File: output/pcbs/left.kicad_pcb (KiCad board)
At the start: 2 copper layers, 132 x 103 mm, 45 parts

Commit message: can't believe that worked
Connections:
- D1 pad 1: (no net) -> P6
- D10 pad 1: (no net) -> P6
- D11 pad 1: (no net) -> P7
- D12 pad 1: (no net) -> P8
- D13 pad 1: (no net) -> P6
- D14 pad 1: (no net) -> P7
- D15 pad 1: (no net) -> P8
- D16 pad 1: (no net) -> P6
- D17 pad 1: (no net) -> P7
- D18 pad 1: (no net) -> P8
- D19 pad 1: (no net) -> P6
- D2 pad 1: (no net) -> P7
- D20 pad 1: (no net) -> P7
- D21 pad 1: (no net) -> P6
- D22 pad 1: (no net) -> P7
- D3 pad 1: (no net) -> P8
- D4 pad 1: (no net) -> P6
- D5 pad 1: (no net) -> P7
- D6 pad 1: (no net) -> P8
- D7 pad 1: (no net) -> P6
- D8 pad 1: (no net) -> P7
- D9 pad 1: (no net) -> P8

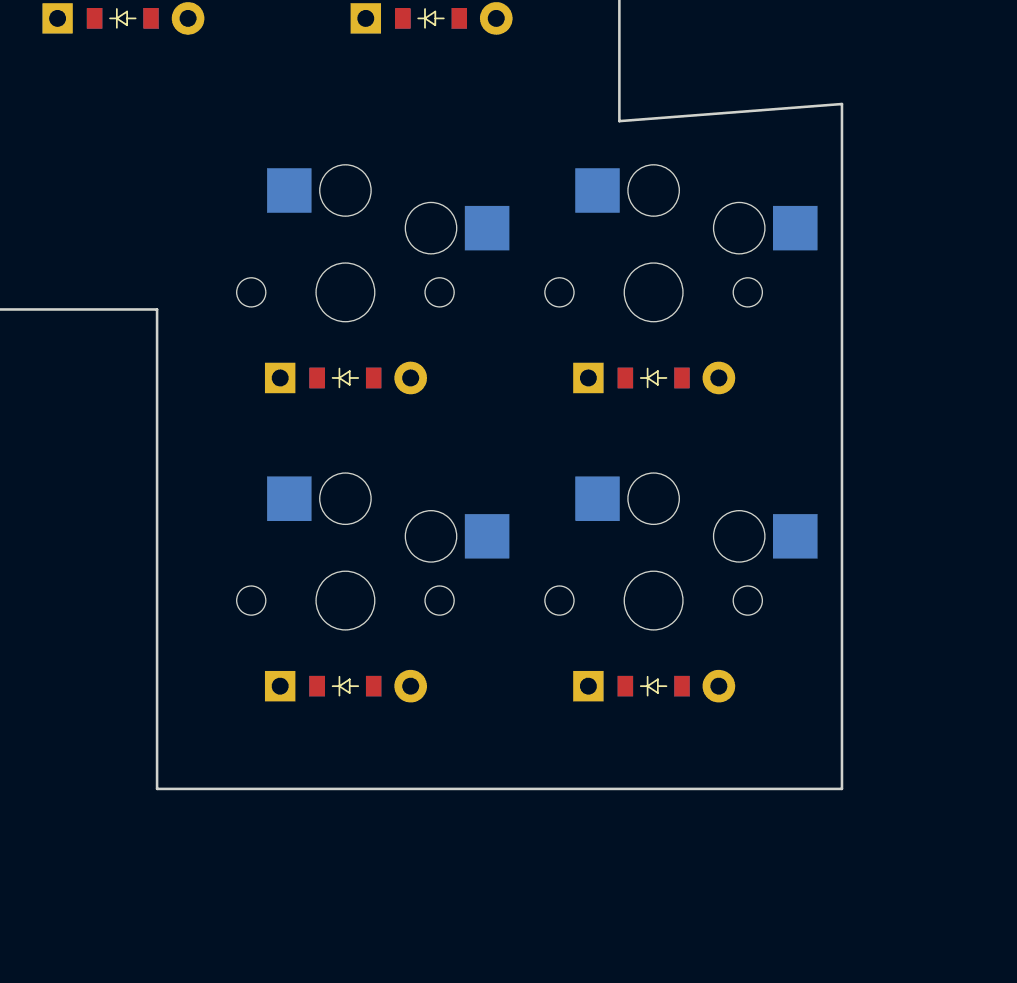
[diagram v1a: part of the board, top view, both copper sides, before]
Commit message: reroute and do some other stuff I honestly forgot
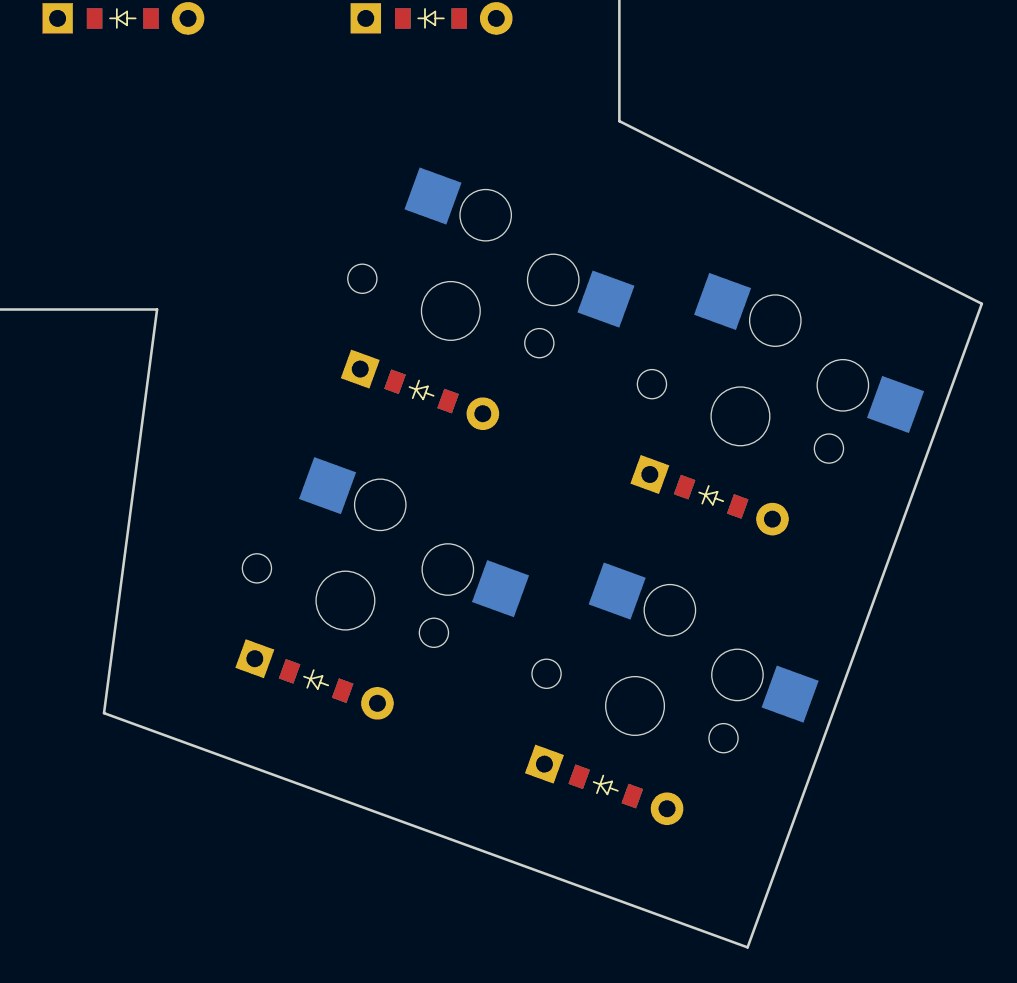
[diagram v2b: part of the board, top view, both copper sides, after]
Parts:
- moved S22 8.84 mm to (108.1, 17.2), turned to -20 degrees
- moved D22 7.71 mm to (106.4, 21.9), turned to -20 degrees
- moved D21 6.49 mm to (100.2, 38.9), turned to -20 degrees
- moved S21 6.25 mm to (101.9, 34.2), turned to -20 degrees
- moved S20 6.25 mm to (91.2, 11.1), turned to -20 degrees
- moved D20 4.51 mm to (89.4, 15.8), turned to -20 degrees
- moved D19 1.74 mm to (83.3, 32.7), turned to -20 degrees
- turned S19 to -20 degrees
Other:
- board size 132 x 103 mm -> 133.2 x 112.3 mm
